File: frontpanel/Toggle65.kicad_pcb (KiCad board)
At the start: 2 copper layers, 144.8 x 94 mm, 122 parts, among them J1 Conn_01x02_Pin, J2 Conn_01x20_Pin, J4 Conn_01x20_Pin, SW10 On-None-Mom, SW11 RUN, SW13 Instruction/Cycle, SW14 RAM or Toggle, SW15 SP3T, SW16 SP3T, SW17 SP3T, SW18 SP3T, SW19 SP3T, SW2 SP3T, SW20 SP3T, SW21 SP3T, SW22 SP3T, SW23 Mom-Off-Mom, SW24 Mom-Off-Mom, SW25 Mom-Off-Mom, SW26 RAM or Toggle, SW27 RAM or Toggle, SW3 SP3T, SW4 SP3T, SW5 SP3T, SW6 SP3T, SW7 SP3T, SW8 SP3T, SW9 SP3T, U2 74HC74

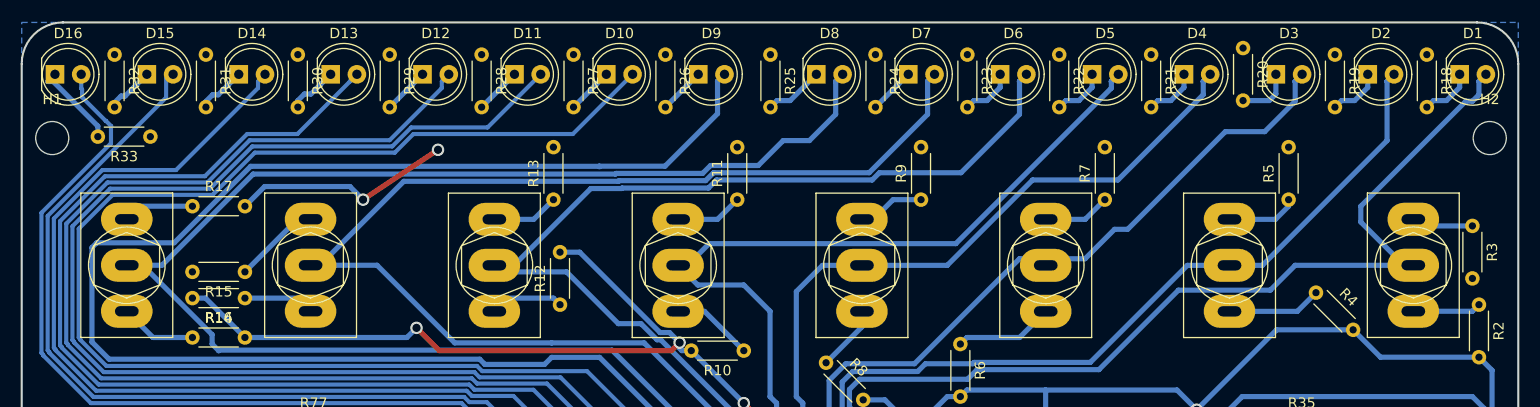
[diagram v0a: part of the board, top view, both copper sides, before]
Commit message: Motherboard finished
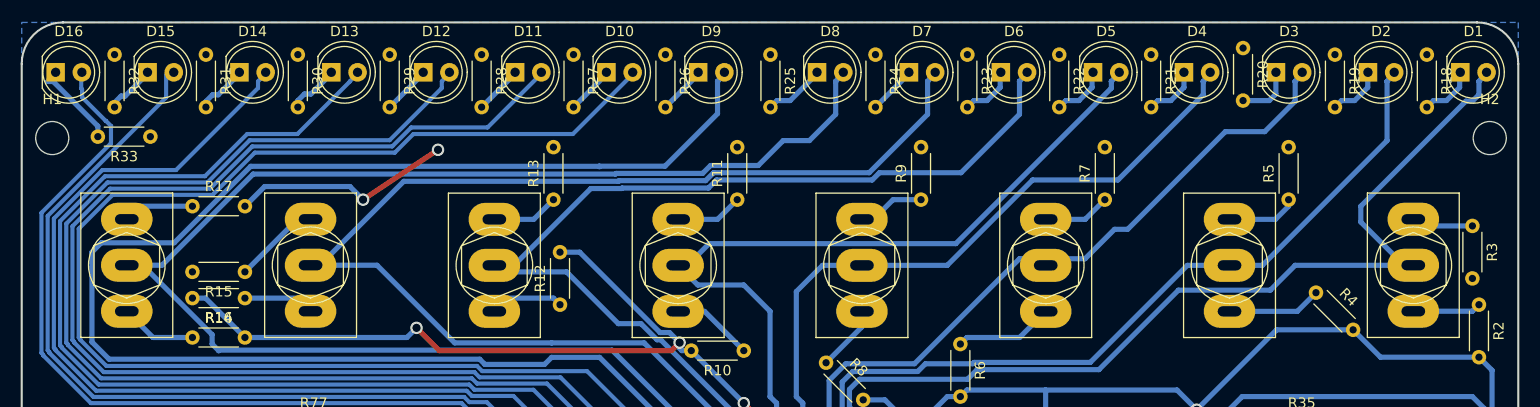
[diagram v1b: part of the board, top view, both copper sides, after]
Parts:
- moved D5 0.22 mm to (126.5, 25.8)
- moved D1 0.20 mm to (162.0, 25.8)
- moved D12 0.20 mm to (61.7, 25.8)
- moved D13 0.20 mm to (52.8, 25.8)
- moved D14 0.20 mm to (43.9, 25.8)
- moved D16 0.20 mm to (26.1, 25.8)
- moved D11 0.20 mm to (70.6, 25.8)
- moved D15 0.20 mm to (35.0, 25.8)
- moved D6 0.20 mm to (117.6, 25.8)
- moved D7 0.20 mm to (108.7, 25.8)
- moved D8 0.20 mm to (99.8, 25.8)
- moved D2 0.19 mm to (153.1, 25.8)
- moved D9 0.19 mm to (88.3, 25.8)
- moved D10 0.19 mm to (79.4, 25.8)
- moved D3 0.19 mm to (144.2, 25.8)
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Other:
- board text added: "Power"
- board text removed: "System"
